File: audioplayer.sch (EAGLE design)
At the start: 16 parts, among them J1 MICRO-SDCARD-CONNECTOR-330006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, J2 JST-2P-SMD-PW-3410050P1, J3 MICRO-USB-5P-340015001, J4 CONNECTOR-HEADER-2X3P-3460180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, J5 AUDIO-CONNECTOR-6P-SMD-344003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, K1 BUTTON-4P-3100010P1, U1 ATMEGA328P-AU-1030060P1, U2 CN3065-1320040P1, U3 XC6206-3.3-1300260P1, U4 LM386M-1100070P1, X1 CRYSTAL-0500290P1

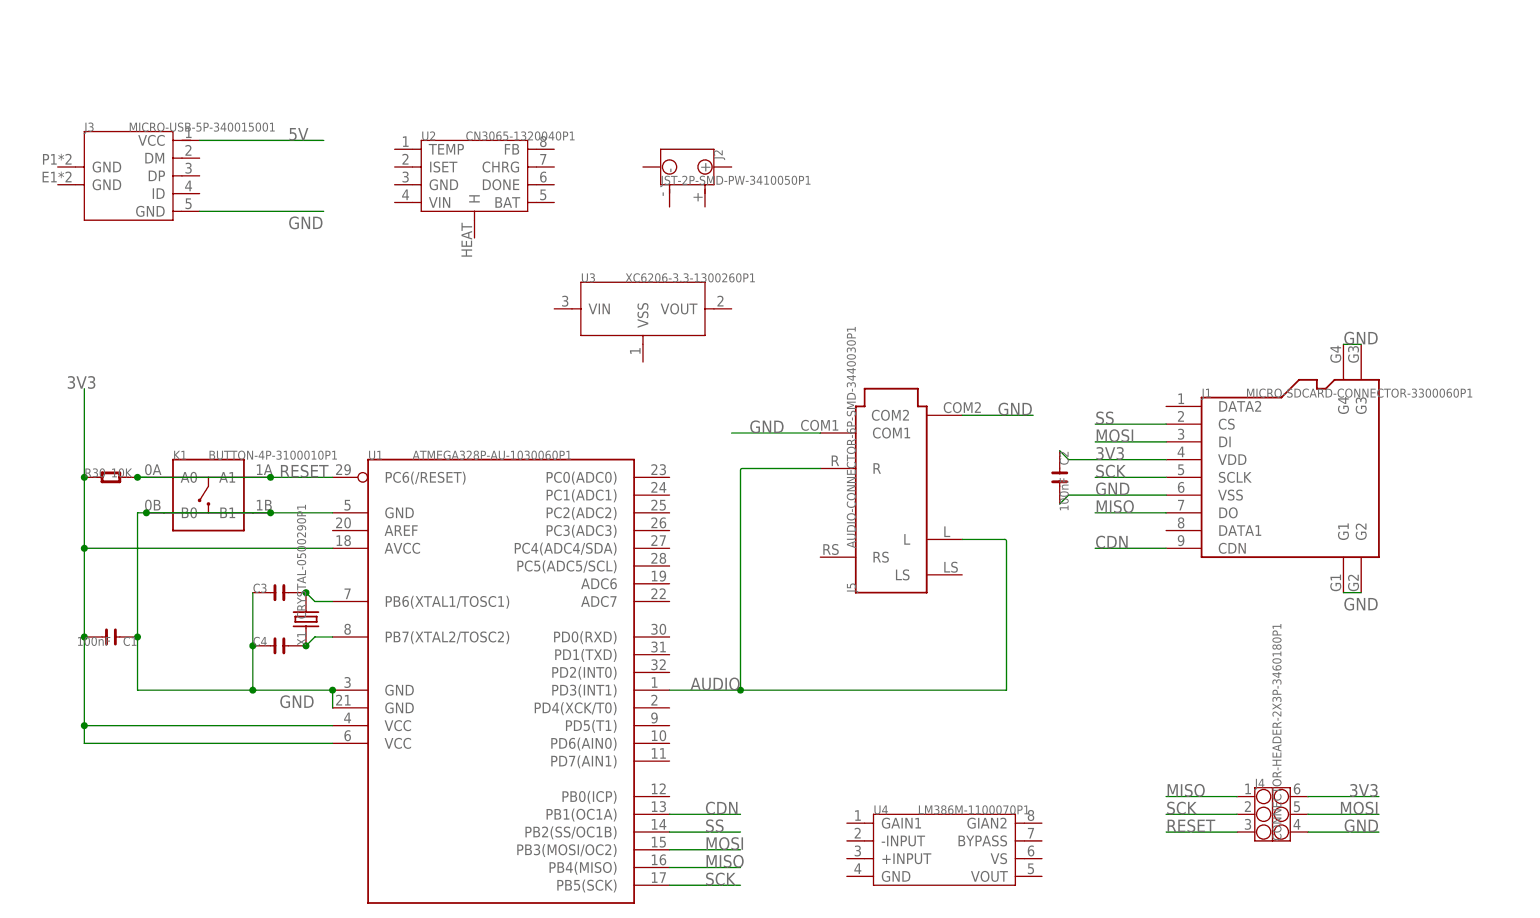
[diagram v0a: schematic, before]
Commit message: 1 hr: Finished basic components and schematic.
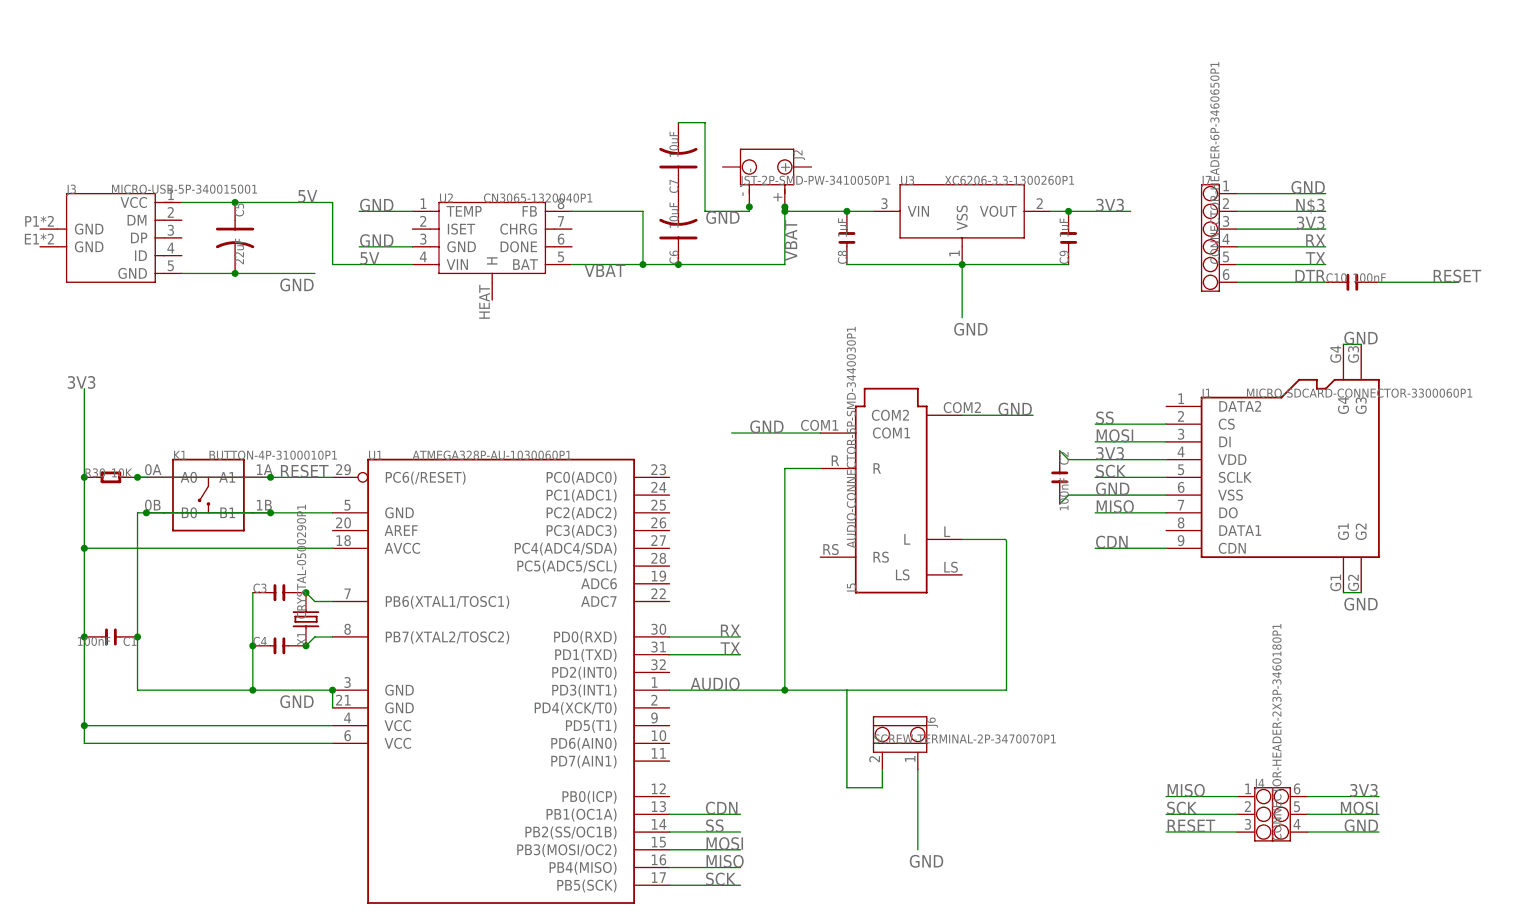
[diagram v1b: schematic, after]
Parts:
- removed U4: LM386M-1100070P1, OPL:LM386M-1100070P1
- added C10: 100nF, OPL:C-0603
- added C5: 22uF, OPL:C-POLAR-B
- added C6, C7: 10uF, OPL:C-POLAR-A
- added C8, C9: 1uF, OPL:C-0805
- added J6: SCREW-TERMINAL-2P-3470070P1, OPL:SCREW-TERMINAL-2P-3470070P1
- added J7: CONNECTOR-HEADER-6P-3460650P1, OPL:CONNECTOR-HEADER-6P-3460650P1
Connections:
- new net DTR: C10.1, J7.6
- new net N$1: C6.2, C7.1
- new net N$3: J7.2
- new net RX: J7.4, U1.PD0(RXD)
- new net TX: J7.5, U1.PD1(TXD)
- new net VBAT: C6.1, C8.2, J2.+, U2.BAT, U2.FB, U3.VIN
- net 3V3: now also C9.2, J7.3, U3.VOUT
- net 5V: now also C5.1, U2.VIN
- net AUDIO: now also J6.2
- net GND: now also C5.2, C7.2, C8.1, C9.1, J2.-, J6.1, J7.1, U2.GND, U2.TEMP, U3.VSS
- net RESET: now also C10.2
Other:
- moved on the sheet: J2, J3, U2, U3
